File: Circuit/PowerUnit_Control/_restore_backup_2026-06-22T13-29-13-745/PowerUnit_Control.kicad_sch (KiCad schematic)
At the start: 25 parts, among them J1 Conn_01x02_Pin, J10 Conn_01x02_Pin, J11 Conn_01x02_Pin, J2 Conn_01x02_Pin, J3 Conn_01x07_Socket, J4 Conn_01x02_Pin, J5 Conn_01x02_Pin, J6 Conn_01x07_Socket, J7 Conn_01x02_Pin, J8 Conn_01x02_Pin, J9 Conn_01x07_Socket, SW1 SW_Toggle_DPDT

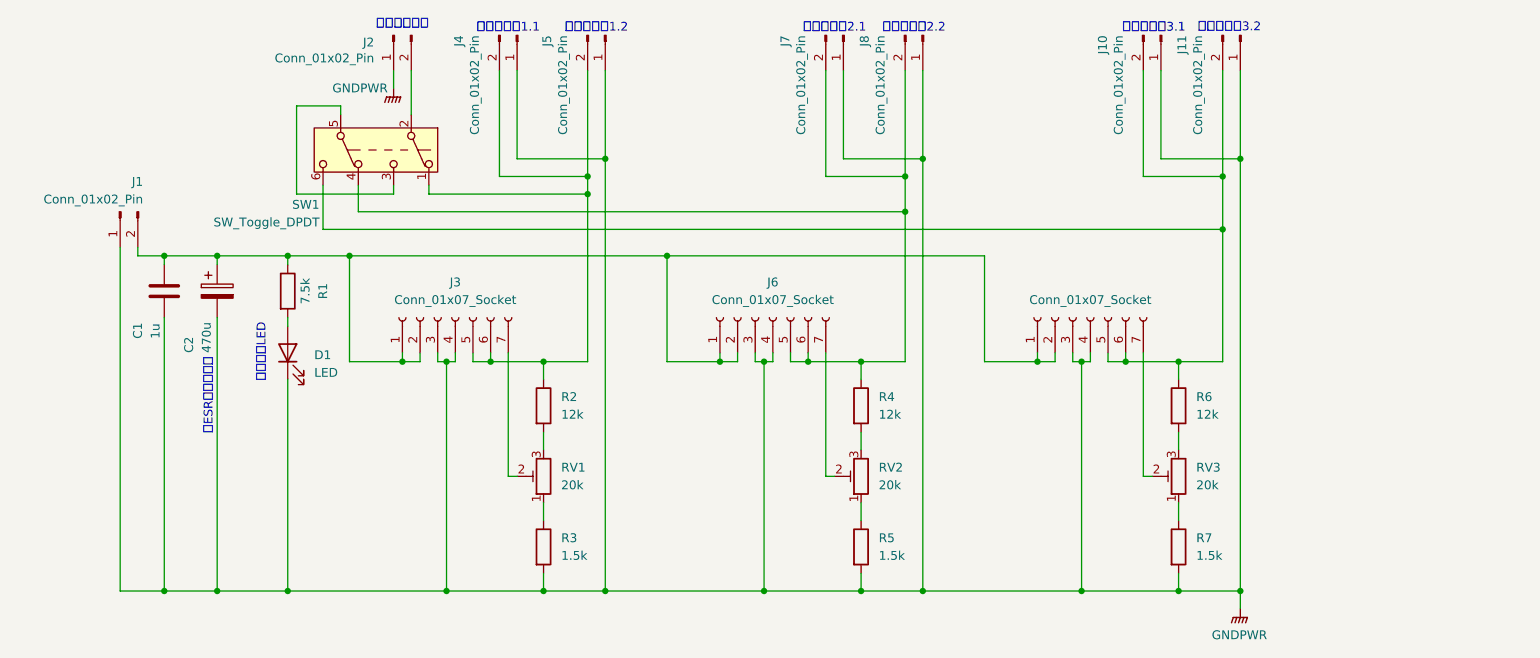
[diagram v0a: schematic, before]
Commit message: 制御電源基板が完成
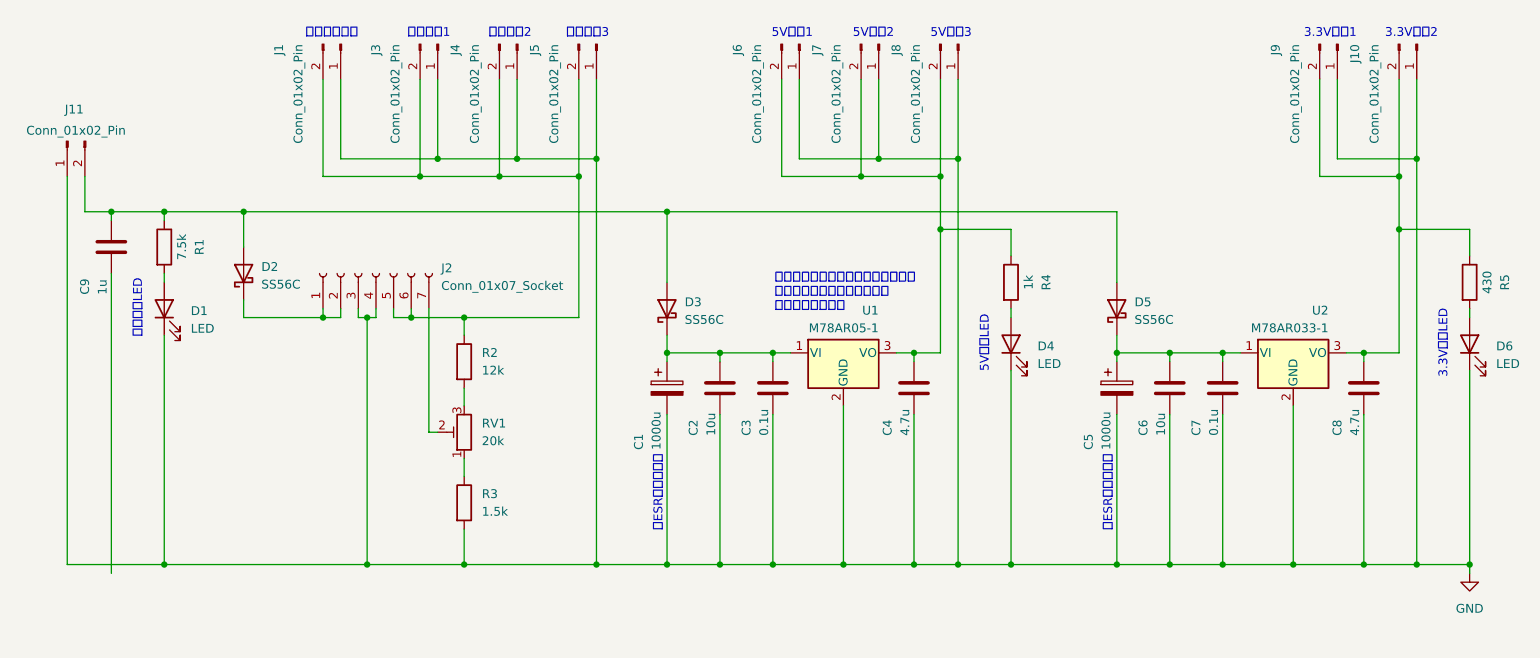
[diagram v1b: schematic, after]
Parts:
- removed C1: 1u, Capacitor_THT:C_Disc_D6.0mm_W4.4mm_P5.00mm, symbol Device:C
- removed C2: 470u, Capacitor_THT:CP_Radial_D10.0mm_P5.00mm, symbol Device:C_Polarized
- removed J2: Conn_01x02_Pin, OU_Conn:Hirose_DF1EC-2P-2.5DSA_1x02_P2.5mm_Vertical, symbol Connector:Conn_01x02_Pin
- removed J3, J6, J9: Conn_01x07_Socket, OU_Power:YDS512F-Unit, symbol Connector:Conn_01x07_Socket
- removed R6: 12k, Resistor_THT:R_Axial_DIN0207_L6.3mm_D2.5mm_P2.54mm_Vertical, symbol Device:R
- removed R7: 1.5k, Resistor_THT:R_Axial_DIN0207_L6.3mm_D2.5mm_P2.54mm_Vertical, symbol Device:R
- removed RV2, RV3: 20k, OU_Reg:TRIM_3296W-1-250, symbol Device:R_Potentiometer_Trim
- removed SW1: SW_Toggle_DPDT, OU_Switch:1MD6-T1-B1-M1-Q-N-S, symbol Switch:SW_Push_DPDT
- added C1, C5: 1000u, Capacitor_THT:CP_Radial_D16.0mm_P7.50mm, symbol Device:C_Polarized
- added C2, C6: 10u, Capacitor_SMD:C_1206_3216Metric, symbol Device:C
- added C3, C7: 0.1u, Capacitor_SMD:C_0603_1608Metric, symbol Device:C
- added C4, C8: 4.7u, Capacitor_SMD:C_0805_2012Metric, symbol Device:C
- added C9: 1u, Capacitor_THT:C_Disc_D6.0mm_W4.4mm_P5.00mm, symbol Device:C
- added D2, D3, D5: SS56C, OU_Diode:DIODE_SS56C-HF_CIP, symbol Device:D_Schottky
- added D4, D6: LED, LED_THT:LED_D5.0mm, symbol Device:LED
- added J2: Conn_01x07_Socket, OU_Power:YDS512F-Unit, symbol Connector:Conn_01x07_Socket
- added J3: Conn_01x02_Pin, OU_Conn:AMASS_XT30U-F, symbol Connector:Conn_01x02_Pin
- added J6, J9: Conn_01x02_Pin, OU_Conn:Hirose_DF1EC-2P-2.5DSA_1x02_P2.5mm_Vertical, symbol Connector:Conn_01x02_Pin
- added U1: M78AR05-1, OU_Power:M78AR05-1, symbol Regulator_Linear:LM7812_TO220
- added U2: M78AR033-1, OU_Power:M78AR033-1, symbol Regulator_Linear:LM7812_TO220
- J1: footprint OU_Conn:AMASS_XT60PW-M -> OU_Conn:Hirose_DF1EC-2P-2.5DSA_1x02_P2.5mm_Vertical
- J10, J7, J8: footprint OU_Conn:AMASS_XT30U-F -> OU_Conn:Hirose_DF1EC-2P-2.5DSA_1x02_P2.5mm_Vertical; MPN XT30PW-M -> (none); MPN_URL https://akizukidenshi.com/catalog/g/g117949/ -> (none)
- J11: footprint OU_Conn:AMASS_XT30U-F -> OU_Conn:AMASS_XT30PW-M
- R2, R3: footprint Resistor_THT:R_Axial_DIN0207_L6.3mm_D2.5mm_P2.54mm_Vertical -> Resistor_SMD:R_0603_1608Metric
- R4: value 12k -> 1k
- R5: value 1.5k -> 430
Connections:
- net at R1.1: now also J11.2 (Pin_2), C9.1, D2.2 (A), D3.2 (A), D5.2 (A); no longer J1.2 (Pin_2)
- net at J10.2 (Pin_2): now also R5.1, C8.1, J9.2 (Pin_2), U2.3 (VO); no longer J11.2 (Pin_2)
- net at J7.2 (Pin_2), J8.2 (Pin_2), R4.1: now also C4.1, J6.2 (Pin_2), U1.3 (VO)
- net at J4.2 (Pin_2), J5.2 (Pin_2), R2.1: now also J1.2 (Pin_2), J2.5 (Pin_5), J2.6 (Pin_6), J3.2 (Pin_2)
- net at R4.2: now also D4.2 (A)
- net at RV1.2: now also J2.7 (Pin_7)
- net GNDPWR renamed GND
- net GND: now also C1.2, C2.2, C3.2, C4.2, C5.2, C6.2, C7.2, C8.2, D4.1 (K), D6.1 (K), J2.3 (Pin_3), J2.4 (Pin_4), J3.1 (Pin_1), J6.1 (Pin_1), J9.1 (Pin_1), U1.2 (GND), U2.2 (GND); no longer R5.2
- new net: C1.1, C2.1, C3.1, D3.1 (K), U1.1 (VI)
- new net: C5.1, C6.1, C7.1, D5.1 (K), U2.1 (VI)
- new net: D2.1 (K), J2.1 (Pin_1), J2.2 (Pin_2)
- new net: D6.2 (A), R5.2
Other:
- note added: "3.3V電源1"
- note added: "3.3V電源2"
- note added: "3.3V電源LED"
- note added: "5V電源1"
- note added: "5V電源2"
- note added: "5V電源3"
- note added: "5V電源LED"
- note added: "リニアレギュレータっぽいですが、 ピン互換があるスイッチング レギュレータです"
- note added: "制御電源LED"
- note added: "汎用電源1"
- note added: "汎用電源2"
- note added: "汎用電源3"
- note removed: "サーボ汎用1.1"
- note removed: "サーボ汎用1.2"
- note removed: "サーボ汎用2.1"
- note removed: "サーボ汎用2.2"
- note removed: "サーボ汎用3.1"
- note removed: "サーボ汎用3.2"
- note removed: "駆動電源LED"
